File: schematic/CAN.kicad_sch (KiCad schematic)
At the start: 7 parts, among them J3 TB006-508-03BE, U2 ISO1050DUBR

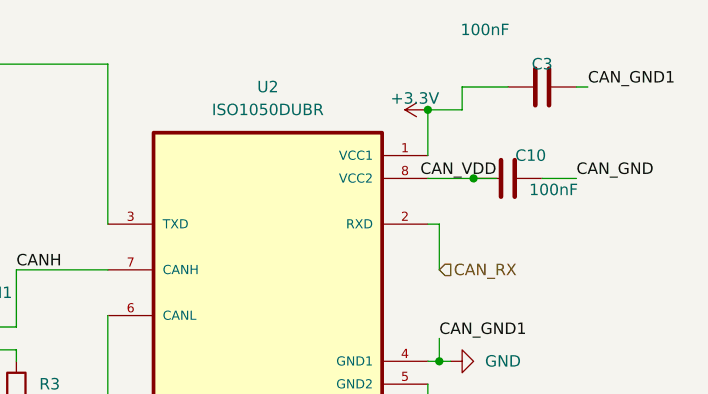
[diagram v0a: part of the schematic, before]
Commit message: Adding Revisions 2 and 3
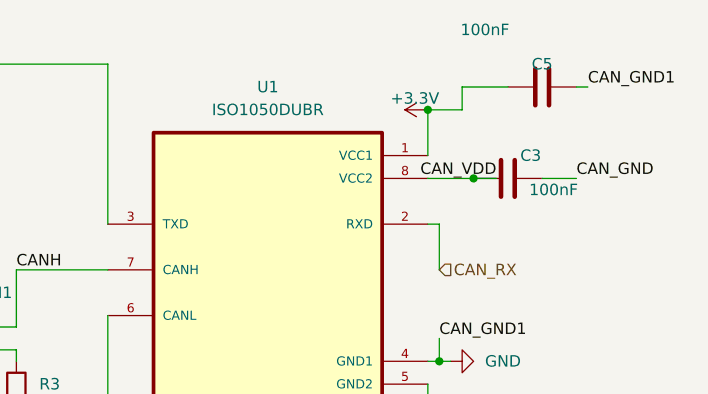
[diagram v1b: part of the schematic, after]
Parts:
- renumbered C10 to C3, C3 to C5, U2 to U1
